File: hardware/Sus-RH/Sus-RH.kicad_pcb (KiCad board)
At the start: 2 copper layers, 47.8 x 62 mm, 46 parts, among them J1 MX150_02x06_Vertical, J2 53307-2471, J4 Conn_01x06, J5 Conn_01x06, U1 TLV9002QDRQ1, U2 LDO40LPURY

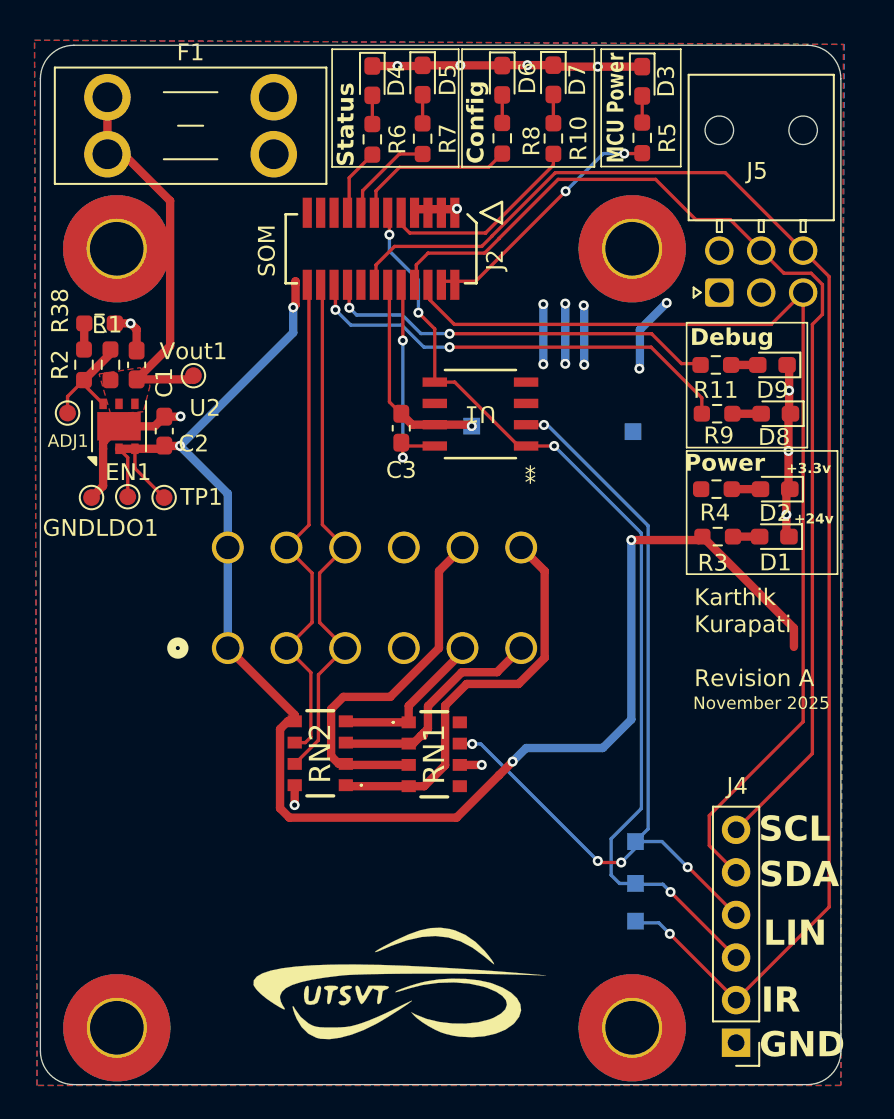
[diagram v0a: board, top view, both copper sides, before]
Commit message: sus rh changes + gerbers
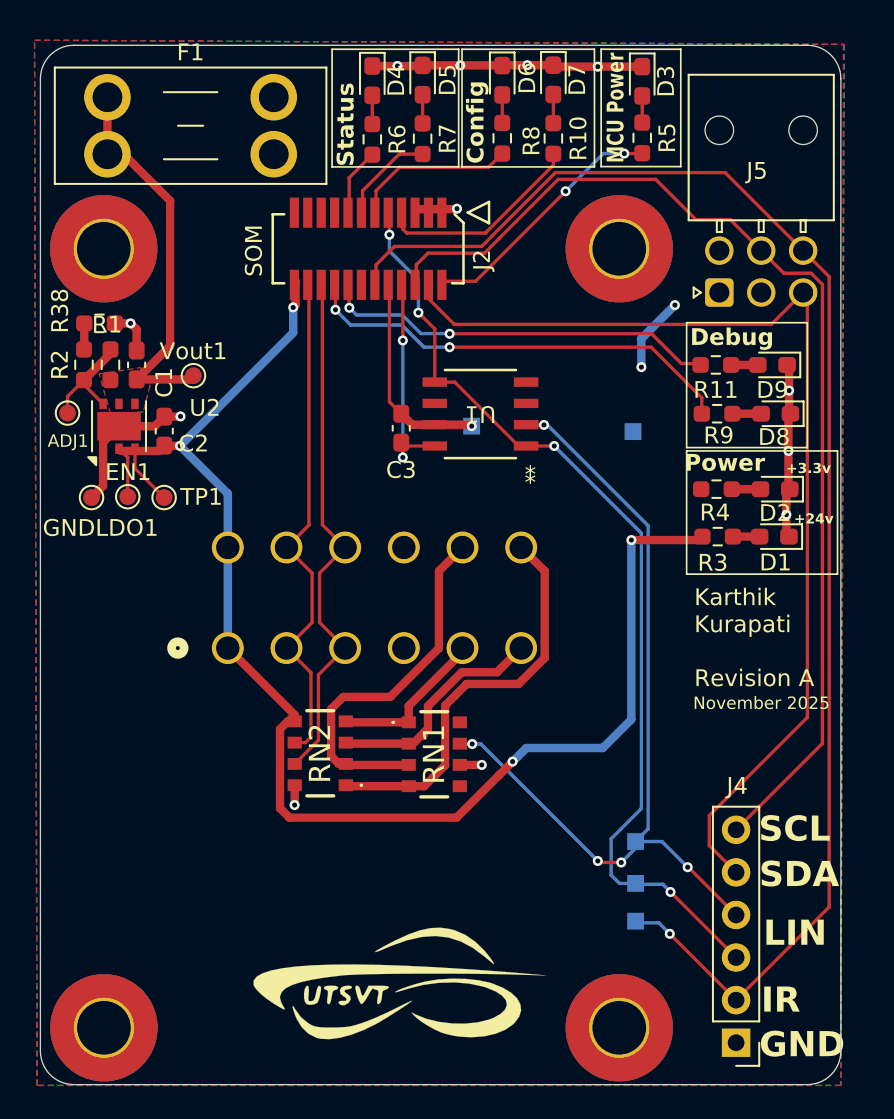
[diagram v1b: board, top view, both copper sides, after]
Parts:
- moved J2 0.77 mm to (85.8, 39.6)
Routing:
- net (no net): track 15.5 -> 0.00 mm, vias 8 -> 0
- net +24V: track 95.8 -> 87.1 mm
- net +3.3V: track 0.00 -> 4.53 mm, vias 0 -> 2
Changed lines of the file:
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@@
 	(footprint "UTSVT_Connectors:PeripheralSOM"
 		(layer "F.Cu")
-		(at 86.57 39.64)
+		(at 85.8 39.64)
 		(property "Reference" "J2"
 			(at 6.8 0.67 90)
@@
 	)
 	(segment
-		(start 96.25 46.57)
-		(end 96.25 46.53)
-		(width 0.5)
-		(layer "F.Cu")
-		(net 0)
-	)
-	(segment
-		(start 102.01 46.76)
-		(end 101.98 46.79)
-		(width 0.5)
-		(layer "F.Cu")
-		(net 0)
-	)
-	(segment
-		(start 98.69 46.62)
-		(end 98.69 46.55)
-		(width 0.5)
-		(layer "F.Cu")
-		(net 0)
-	)
-	(via
-		(at 98.66 43.02)
-		(size 0.6)
-		(drill 0.3)
-		(layers "F.Cu" "B.Cu")
-		(net 0)
-	)
-	(via
-		(at 96.25 46.53)
-		(size 0.6)
-		(drill 0.3)
-		(layers "F.Cu" "B.Cu")
-		(net 0)
-	)
-	(via
-		(at 98.69 46.55)
-		(size 0.6)
-		(drill 0.3)
-		(layers "F.Cu" "B.Cu")
-		(net 0)
-	)
-	(via
-		(at 97.56 42.91)
-		(size 0.6)
-		(drill 0.3)
-		(layers "F.Cu" "B.Cu")
-		(net 0)
-	)
-	(via
-		(at 97.56 46.5)
-		(size 0.6)
-		(drill 0.3)
-		(layers "F.Cu" "B.Cu")
-		(net 0)
-	)
-	(via
-		(at 103.61 42.87)
-		(size 0.6)
-		(drill 0.3)
-		(layers "F.Cu" "B.Cu")
-		(net 0)
-	)
-	(via
-		(at 96.25 42.95)
-		(size 0.6)
-		(drill 0.3)
-		(layers "F.Cu" "B.Cu")
-		(net 0)
-	)
-	(via
-		(at 101.98 46.79)
-		(size 0.6)
-		(drill 0.3)
-		(layers "F.Cu" "B.Cu")
-		(net 0)
-	)
-	(segment
-		(start 102.01 44.47)
-		(end 103.61 42.87)
-		(width 0.5)
-		(layer "B.Cu")
-		(net 0)
-	)
-	(segment
-		(start 97.56 46.5)
-		(end 97.56 42.91)
-		(width 0.5)
-		(layer "B.Cu")
-		(net 0)
-	)
-	(segment
-		(start 98.69 46.55)
-		(end 98.69 43.05)
-		(width 0.5)
-		(layer "B.Cu")
-		(net 0)
-	)
-	(segment
-		(start 101.98 46.79)
-		(end 102.01 46.76)
-		(width 0.5)
-		(layer "B.Cu")
-		(net 0)
-	)
-	(segment
-		(start 102.01 46.76)
-		(end 102.01 44.47)
-		(width 0.5)
-		(layer "B.Cu")
-		(net 0)
-	)
-	(segment
-		(start 96.25 46.53)
-		(end 96.25 42.95)
-		(width 0.5)
-		(layer "B.Cu")
-		(net 0)
-	)
-	(segment
-		(start 98.69 43.05)
-		(end 98.66 43.02)
-		(width 0.5)
-		(layer "B.Cu")
-		(net 0)
-	)
-	(segment
 		(start 96.9375 28.775)
 		(end 96.85 28.6875)
@@
 		(net 1)
 	)
+	(via
+		(at 104.1 43)
+		(size 0.6)
+		(drill 0.3)
+		(layers "F.Cu" "B.Cu")
+		(free yes)
+		(net 2)
+	)
+	(via
+		(at 102.1 46.7)
+		(size 0.6)
+		(drill 0.3)
+		(layers "F.Cu" "B.Cu")
+		(free yes)
+		(net 2)
+	)
+	(segment
+		(start 102.1 45)
+		(end 104.1 43)
+		(width 0.5)
+		(layer "B.Cu")
+		(net 2)
+	)
+	(segment
+		(start 102.1 46.7)
+		(end 102.1 45)
+		(width 0.5)
+		(layer "B.Cu")
+		(net 2)
+	)
 	(segment
 		(start 81.47 43)
@@
 	)
 	(segment
-		(start 70.94 51.57)
-		(end 73.45 51.57)
-		(width 0.5)
-		(layer "F.Cu")
-		(net 3)
-	)
-	(segment
 		(start 91.077005 73.574995)
 		(end 81.102925 73.574995)
@@
 	)
 	(segment
-		(start 105.74125 56.81)
-		(end 111.199 62.26775)
+		(start 71.07 51.7)
+		(end 73.32 51.7)
 		(width 0.5)
 		(layer "F.Cu")
@@
 	)
 	(segment
-		(start 111.199 62.26775)
-		(end 111.199 63.39)
-		(width 0.5)
-		(layer "F.Cu")
-		(net 3)
-	)
-	(segment
 		(start 93.609265 71.040735)
 		(end 93.609265 71.042735)
@@
 	)
 	(segment
-		(start 73.45 51.57)
-		(end 73.64 51.38)
-		(width 0.5)
+		(start 71.89 51.57)
+		(end 71.89 52.74)
+		(width 0.2)
 		(layer "F.Cu")
 		(net 3)
 	)
 	(segment
-		(start 71.89 51.57)
-		(end 71.89 52.74)
-		(width 0.2)
+		(start 73.32 51.7)
+		(end 73.64 51.38)
+		(width 0.5)
 		(layer "F.Cu")
 		(net 3)
@@
 		(net 3)
 	)
+	(segment
+		(start 70.94 51.57)
+		(end 71.07 51.7)
+		(width 0.5)
+		(layer "F.Cu")
+		(net 3)
+	)
 	(via
 		(at 101.5 57.016765)
@@
 	(segment
 		(start 111.75 42.25)
-		(end 109.85 44.15)
+		(end 112 42.5)
 		(width 0.2)
 		(layer "F.Cu")
@@
 	)
 	(segment
-		(start 109.85 44.15)
-		(end 90.94 44.15)
+		(start 112 67.6)
+		(end 106.15 73.45)
 		(width 0.2)
 		(layer "F.Cu")
@@
 	(segment
 		(start 111.75 42.25)
-		(end 111.75 67.85)
+		(end 109.85 44.15)
+		(width 0.2)
+		(layer "F.Cu")
+		(net 18)
+	)
+	(segment
+		(start 109.85 44.15)
+		(end 90.94 44.15)
 		(width 0.2)
 		(layer "F.Cu")
@@
 	)
 	(segment
-		(start 111.75 67.85)
-		(end 106.15 73.45)
+		(start 106.15 73.45)
+		(end 106.15 75.24)
 		(width 0.2)
 		(layer "F.Cu")
@@
 	)
 	(segment
-		(start 106.15 73.45)
-		(end 106.15 75.24)
+		(start 112 42.5)
+		(end 112 67.6)
 		(width 0.2)
 		(layer "F.Cu")
@@
 	)
 	(segment
-		(start 88.28 38.7)
-		(end 92.81 38.7)
+		(start 87.87 38.47)
+		(end 88.1 38.7)
 		(width 0.2)
 		(layer "F.Cu")
@@
 	)
 	(segment
-		(start 87.87 38.29)
-		(end 88.28 38.7)
+		(start 87.87 37.28)
+		(end 87.87 38.47)
 		(width 0.2)
 		(layer "F.Cu")
@@
 	)
 	(segment
-		(start 87.87 37.28)
-		(end 87.87 38.29)
+		(start 92.81 38.7)
+		(end 92.81 38.69)
 		(width 0.2)
 		(layer "F.Cu")
@@
 	)
 	(segment
-		(start 92.81 38.69)
-		(end 96.85 34.65)
+		(start 88.1 38.7)
+		(end 92.81 38.7)
 		(width 0.2)
 		(layer "F.Cu")
@@
 	)
 	(segment
-		(start 92.81 38.7)
-		(end 92.81 38.69)
+		(start 92.81 38.69)
+		(end 96.85 34.65)
 		(width 0.2)
 		(layer "F.Cu")
@@
 	)
 	(segment
-		(start 112.3 69.75)
+		(start 112.901 69.149)
 		(end 107.75 74.3)
 		(width 0.2)
@@
 	)
 	(segment
-		(start 112.901 41.77324)
-		(end 112.901 43.549)
+		(start 110.599 41.099)
+		(end 112.22676 41.099)
 		(width 0.2)
 		(layer "F.Cu")
@@
 	)
 	(segment
-		(start 110.599 41.099)
-		(end 112.22676 41.099)
-		(width 0.2)
-		(layer "F.Cu")
-		(net 40)
-	)
-	(segment
-		(start 109.25 39.75)
-		(end 110.599 41.099)
-		(width 0.2)
-		(layer "F.Cu")
-		(net 40)
-	)
-	(segment
 		(start 89.373 39.9)
 		(end 92.7442 39.9)
@@
 	)
 	(segment
-		(start 112.901 43.549)
-		(end 112.3 44.15)
+		(start 92.7442 39.9)
+		(end 93.612 39.0322)
 		(width 0.2)
 		(layer "F.Cu")
@@
 	)
 	(segment
-		(start 92.7442 39.9)
-		(end 93.612 39.0322)
+		(start 112.901 41.77324)
+		(end 112.901 69.149)
 		(width 0.2)
 		(layer "F.Cu")
@@
 	)
 	(segment
-		(start 112.3 44.15)
-		(end 112.3 69.75)
+		(start 109.25 39.75)
+		(end 110.599 41.099)
 		(width 0.2)
 		(layer "F.Cu")
